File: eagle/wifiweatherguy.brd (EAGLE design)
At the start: 100 x 80 mm, 3 parts

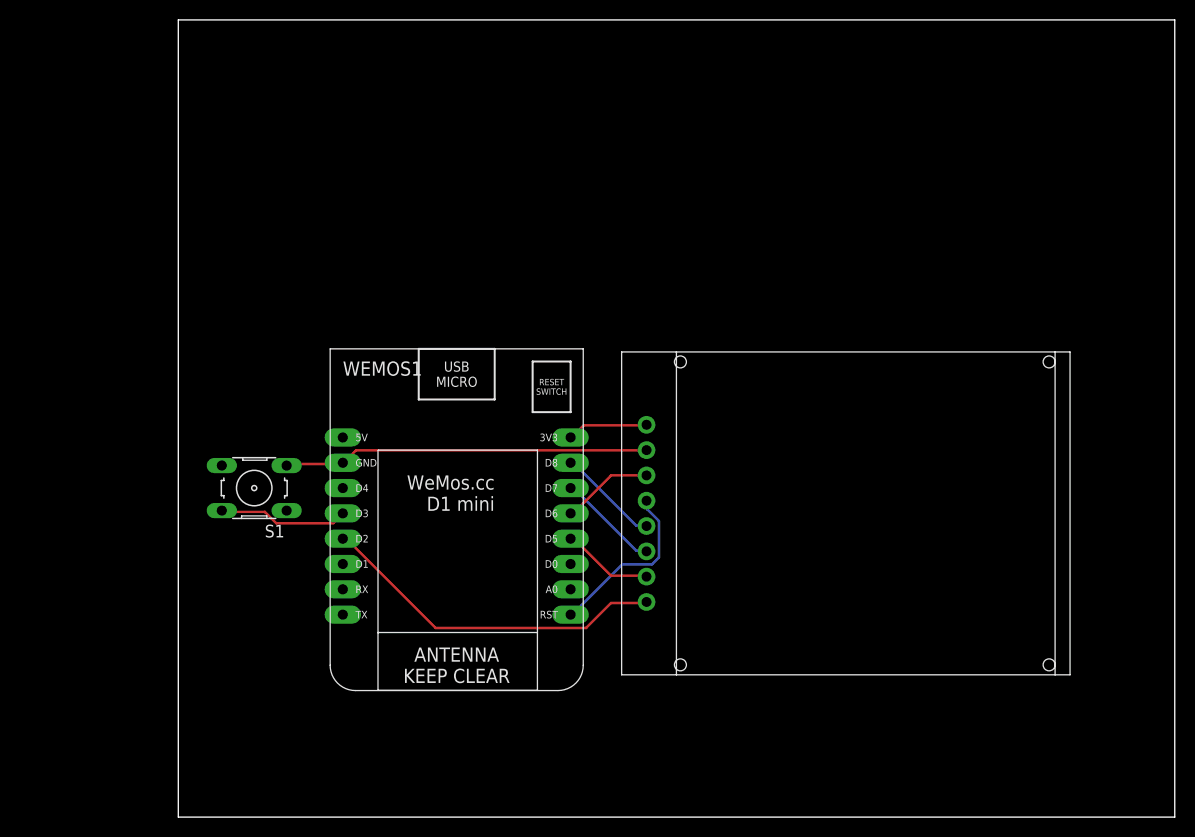
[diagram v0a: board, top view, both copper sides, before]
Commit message: update layout
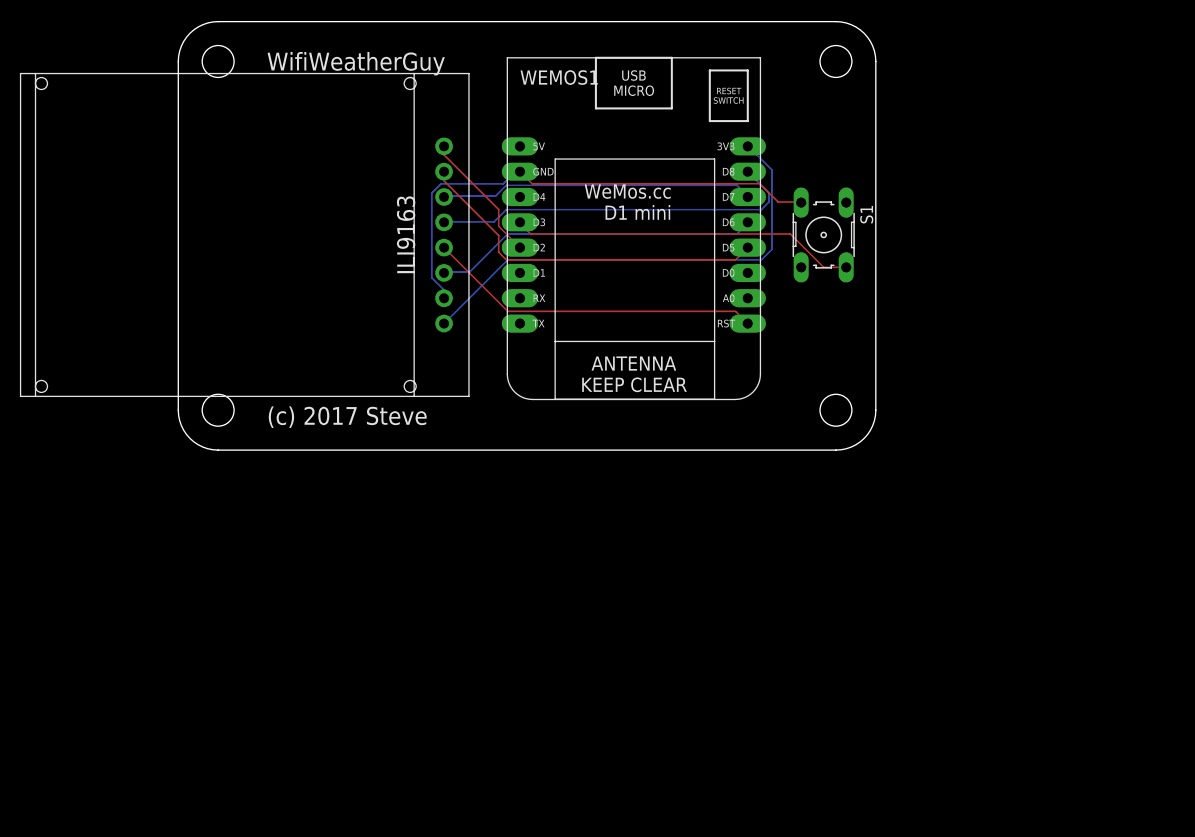
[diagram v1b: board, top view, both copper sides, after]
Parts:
- added U$2: (no value), dp_pcb:DP7043_V1
- moved S1 62.5 mm to (64.8, 58.4), turned to 270 degrees
- moved U$1 50.0 mm to (26.7, 67.3), turned to 180 degrees
- moved WEMOS1 34.2 mm to (47.0, 57.1)
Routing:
- net N$1: track 8.12 -> 47.4 mm
- net N$3: track 10.3 -> 37.4 mm
- net N$5: track 9.34 -> 36.2 mm
- net N$2: track 9.25 -> 32.7 mm
- net N$6: track 35.4 -> 13.3 mm
- net N$9: track 13.1 -> 34.7 mm
- net N$4: track 10.3 -> 31.6 mm
- net N$8: track 17.4 -> 33.6 mm
- net N$7: track 36.8 -> 50.3 mm
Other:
- board size 100 x 80 mm -> 70 x 43 mm
- board text added: "(c) 2017 Steve"
- board text added: "ILI9163"
- board text added: "WifiWeatherGuy"
